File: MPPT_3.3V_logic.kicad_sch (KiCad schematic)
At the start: 11 parts, among them Q1 PMOS, Q2 PMOS, U1 LTC4412xS6, U2 TPS62177DQCR, U3 LTC4412xS6

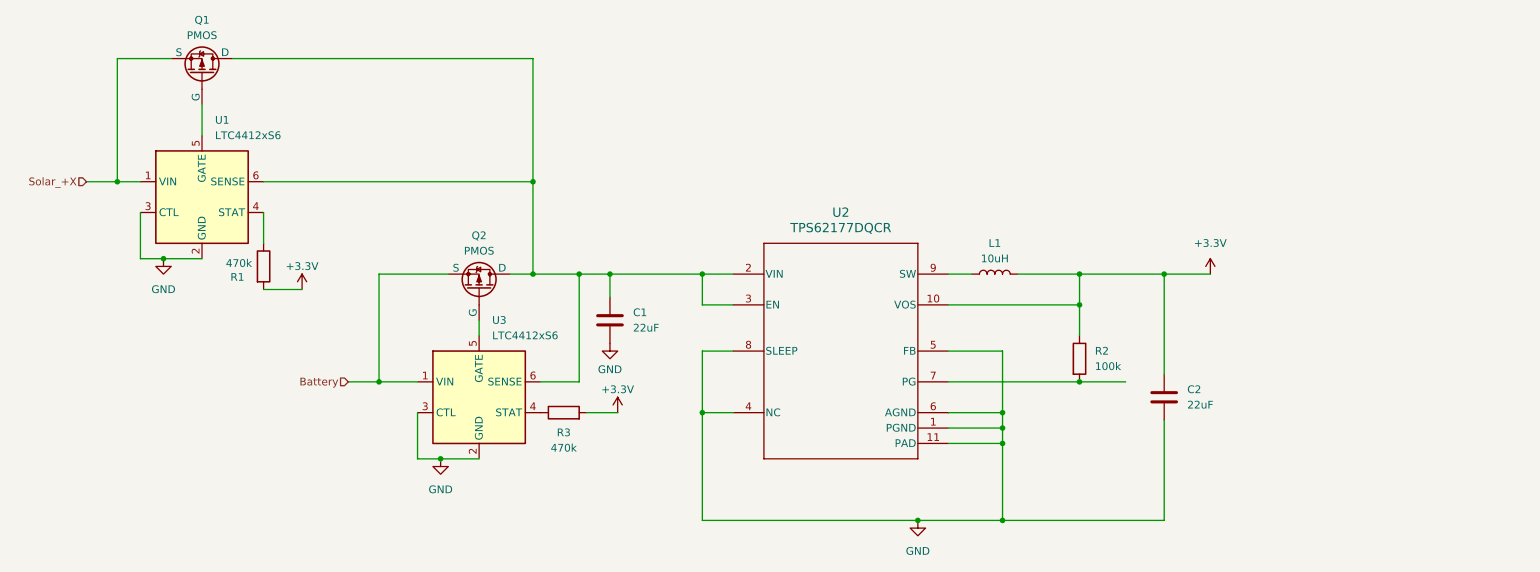
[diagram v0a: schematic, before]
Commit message: Added footprints to caps
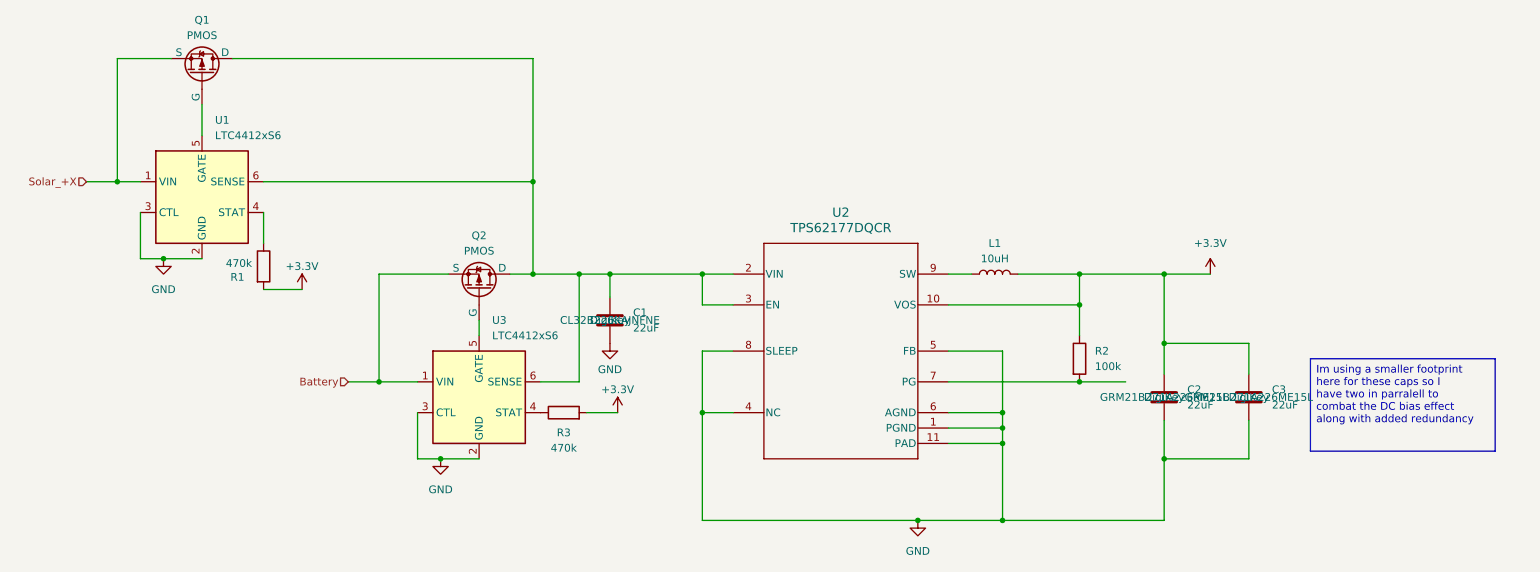
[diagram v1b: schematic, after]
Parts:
- added C3: 22uF, Capacitor_SMD:C_0805_2012Metric, symbol Device:C
- C1: footprint (none) -> Capacitor_SMD:C_1210_3225Metric; MANUFACTURER (none) -> DigiKey; MANUFACTURER_PART_NUMBER (none) -> CL32B226KAJNFNE
- C2: footprint (none) -> Capacitor_SMD:C_0805_2012Metric; MANUFACTURER (none) -> DigiKey; MANUFACTURER_PART_NUMBER (none) -> GRM21BZ71A226ME15L
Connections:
- net +3.3V: now also C3.1
- net GND: now also C3.2
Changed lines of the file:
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@@
 		(company "QSET (Jaron Cyna)")
+	)
+	(text_box "Im using a smaller footprint here for these caps so I have two in parralell to combat the DC bias effect along with added redundancy"
+		(exclude_from_sim no)
+		(at 251.46 104.14 0)
+		(size 30.48 15.24)
+		(margins 0.9525 0.9525 0.9525 0.9525)
+		(stroke
+			(width 0)
+			(type solid)
+		)
+		(fill
+			(type color)
+			(color 158 218 255 1)
+		)
+		(effects
+			(font
+				(size 1.27 1.27)
+			)
+			(justify left top)
+		)
 	)
 	(junction
@@
 	)
 	(junction
+		(at 227.33 101.6)
+		(diameter 0)
+		(color 0 0 0 0)
+	)
+	(junction
+		(at 227.33 120.65)
+		(diameter 0)
+		(color 0 0 0 0)
+	)
+	(junction
 		(at 227.33 90.17)
 		(diameter 0)
@@
 	(wire
 		(pts
+			(xy 227.33 101.6) (xy 241.3 101.6)
+		)
+		(stroke
+			(width 0)
+			(type default)
+		)
+	)
+	(wire
+		(pts
 			(xy 68.58 62.23) (xy 68.58 67.31)
 		)
@@
 	(wire
 		(pts
+			(xy 241.3 101.6) (xy 241.3 106.68)
+		)
+		(stroke
+			(width 0)
+			(type default)
+		)
+	)
+	(wire
+		(pts
 			(xy 191.77 95.25) (xy 213.36 95.25)
 		)
@@
 	(wire
 		(pts
+			(xy 227.33 120.65) (xy 241.3 120.65)
+		)
+		(stroke
+			(width 0)
+			(type default)
+		)
+	)
+	(wire
+		(pts
 			(xy 124.46 107.95) (xy 130.81 107.95)
 		)
@@
 	(wire
 		(pts
-			(xy 227.33 90.17) (xy 227.33 106.68)
-		)
-		(stroke
-			(width 0)
-			(type default)
-		)
-	)
-	(wire
-		(pts
 			(xy 135.89 90.17) (xy 135.89 93.98)
 		)
@@
 	(wire
 		(pts
+			(xy 227.33 90.17) (xy 227.33 101.6)
+		)
+		(stroke
+			(width 0)
+			(type default)
+		)
+	)
+	(wire
+		(pts
 			(xy 200.66 130.81) (xy 227.33 130.81)
 		)
@@
 	(wire
 		(pts
+			(xy 241.3 120.65) (xy 241.3 114.3)
+		)
+		(stroke
+			(width 0)
+			(type default)
+		)
+	)
+	(wire
+		(pts
+			(xy 227.33 101.6) (xy 227.33 106.68)
+		)
+		(stroke
+			(width 0)
+			(type default)
+		)
+	)
+	(wire
+		(pts
 			(xy 78.74 74.93) (xy 123.19 74.93)
 		)
@@
 	(wire
 		(pts
+			(xy 227.33 120.65) (xy 227.33 130.81)
+		)
+		(stroke
+			(width 0)
+			(type default)
+		)
+	)
+	(wire
+		(pts
 			(xy 191.77 102.87) (xy 200.66 102.87)
 		)
@@
 	(wire
 		(pts
-			(xy 227.33 114.3) (xy 227.33 130.81)
+			(xy 227.33 114.3) (xy 227.33 120.65)
 		)
 		(stroke
@@
 			)
 		)
-		(property "Footprint" ""
+		(property "Footprint" "Capacitor_SMD:C_1210_3225Metric"
 			(at 136.8552 101.6 0)
 			(effects
@@
 			)
 		)
-		(property "Datasheet" "~"
+		(property "Datasheet" "https://mm.digikey.com/Volume0/opasdata/d220001/medias/docus/2113/CL32B226KAJNFNE_Spec.pdf"
 			(at 135.89 97.79 0)
 			(effects
@@
 				)
 				(hide yes)
+			)
+		)
+		(property "MANUFACTURER" "DigiKey"
+			(at 135.89 97.79 0)
+			(effects
+				(font
+					(size 1.27 1.27)
+				)
+			)
+		)
+		(property "MANUFACTURER_PART_NUMBER" "CL32B226KAJNFNE"
+			(at 135.89 97.79 0)
+			(effects
+				(font
+					(size 1.27 1.27)
+				)
 			)
 		)
@@
 	)
 	(symbol
+		(lib_id "Device:C")
+		(at 241.3 110.49 0)
+		(unit 1)
+		(exclude_from_sim no)
+		(in_bom yes)
+		(on_board yes)
+		(dnp no)
+		(fields_autoplaced yes)
+		(property "Reference" "C3"
+			(at 245.11 109.2199 0)
+			(effects
+				(font
+					(size 1.27 1.27)
+				)
+				(justify left)
+			)
+		)
+		(property "Value" "22uF"
+			(at 245.11 111.7599 0)
+			(effects
+				(font
+					(size 1.27 1.27)
+				)
+				(justify left)
+			)
+		)
+		(property "Footprint" "Capacitor_SMD:C_0805_2012Metric"
+			(at 242.2652 114.3 0)
+			(effects
+				(font
+					(size 1.27 1.27)
+				)
+				(hide yes)
+			)
+		)
+		(property "Datasheet" "https://search.murata.co.jp/Ceramy/image/img/A01X/G101/ENG/GRM21BZ71A226ME15-01.pdf"
+			(at 241.3 110.49 0)
+			(effects
+				(font
+					(size 1.27 1.27)
+				)
+				(hide yes)
+			)
+		)
+		(property "Description" "Unpolarized capacitor"
+			(at 241.3 110.49 0)
+			(effects
+				(font
+					(size 1.27 1.27)
+				)
+				(hide yes)
+			)
+		)
+		(property "MANUFACTURER" "DigiKey"
+			(at 241.3 110.49 0)
+			(effects
+				(font
+					(size 1.27 1.27)
+				)
+			)
+		)
+		(property "MANUFACTURER_PART_NUMBER" "GRM21BZ71A226ME15L"
+			(at 241.3 110.49 0)
+			(effects
+				(font
+					(size 1.27 1.27)
+				)
+			)
+		)
+		(pin "1"
+		)
+		(pin "2"
+		)
+		(instances
+			(project "EPS_mppt_board"
+				(path "/8f246f89-1ec7-4136-9977-839b50e116ed/1cb04f15-5cd4-4c9d-a391-62735eda9253"
+					(reference "C3")
+					(unit 1)
+				)
+			)
+		)
+	)
+	(symbol
 		(lib_id "power:GND")
 		(at 135.89 101.6 0)
@@
 			)
 		)
-		(property "Footprint" ""
+		(property "Footprint" "Capacitor_SMD:C_0805_2012Metric"
 			(at 228.2952 114.3 0)
 			(effects
@@
 			)
 		)
-		(property "Datasheet" "~"
+		(property "Datasheet" "https://search.murata.co.jp/Ceramy/image/img/A01X/G101/ENG/GRM21BZ71A226ME15-01.pdf"
 			(at 227.33 110.49 0)
 			(effects
@@
 			)
 		)
+		(property "MANUFACTURER" "DigiKey"
+			(at 227.33 110.49 0)
+			(effects
+				(font
+					(size 1.27 1.27)
+				)
+			)
+		)
+		(property "MANUFACTURER_PART_NUMBER" "GRM21BZ71A226ME15L"
+			(at 227.33 110.49 0)
+			(effects
+				(font
+					(size 1.27 1.27)
+				)
+			)
+		)
